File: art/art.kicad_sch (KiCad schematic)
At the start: 14 parts, among them J1 AudioJack4, SW1 SW_Push, SW2 SW_Push, SW3 SW_Push, SW4 SW_Push, SW5 SW_Push, SW6 SW_Push, SW7 SW_Push, SW8 SW_Push, U1 rp2040-zero

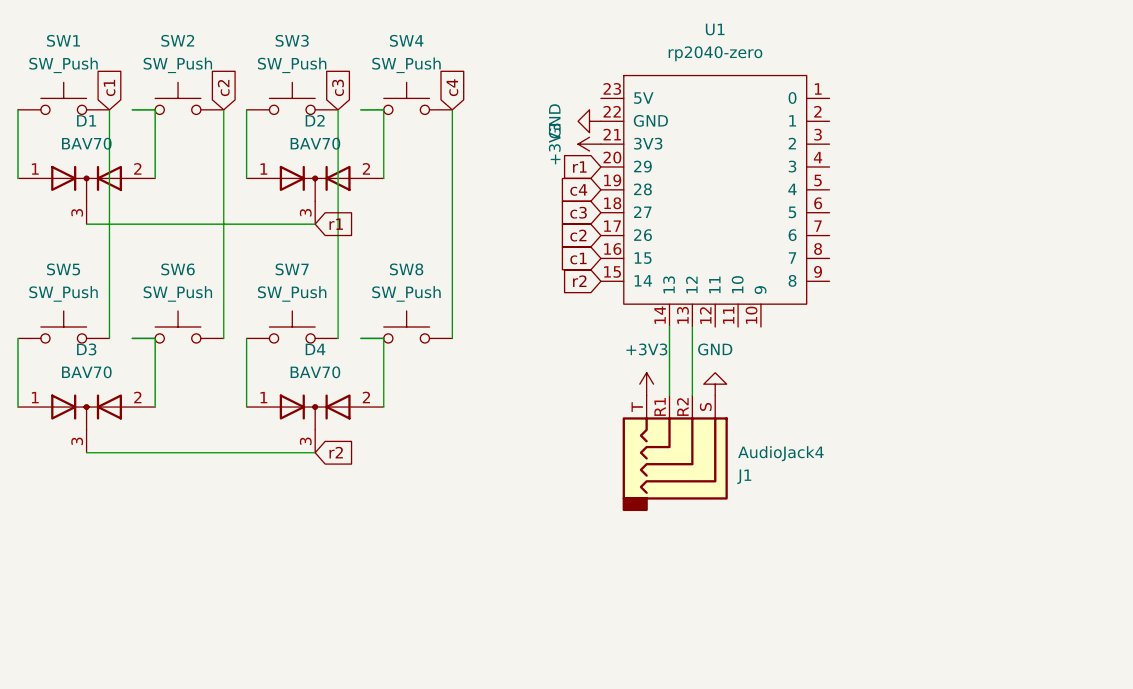
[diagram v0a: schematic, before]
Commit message: .
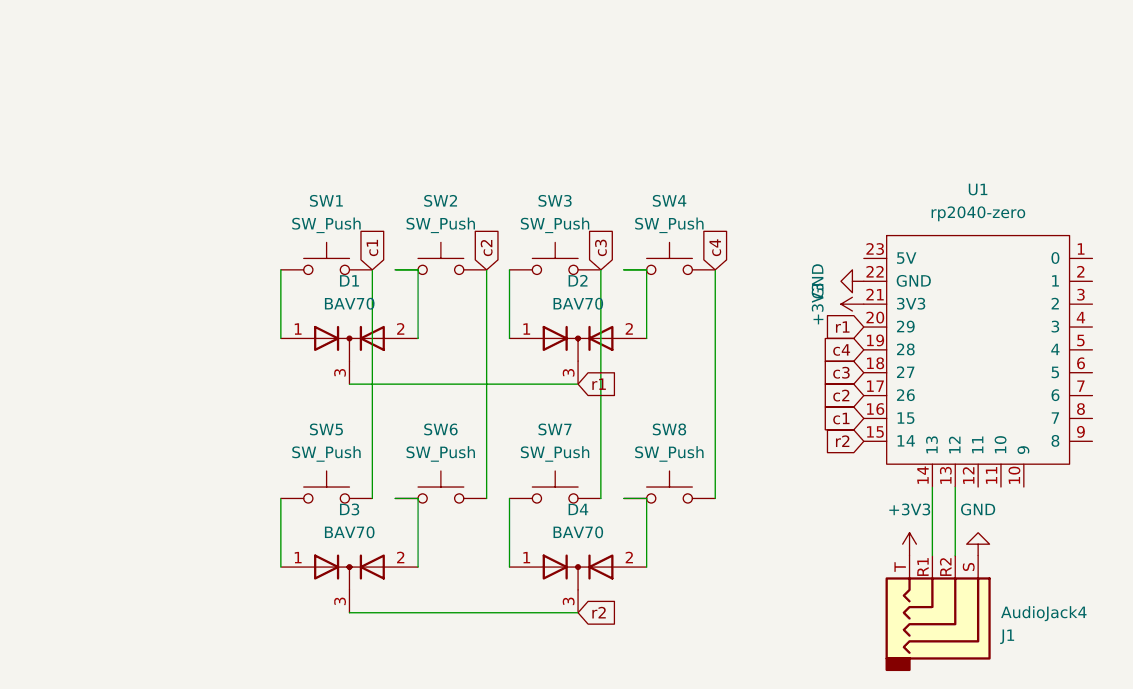
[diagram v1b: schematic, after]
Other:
- title: (none) -> Art Pad
- moved on the sheet: D1, D2, D3, D4, J1, SW1, SW2, SW3, SW4, SW5, SW6, SW7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
